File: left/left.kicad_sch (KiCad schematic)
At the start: 19 parts, among them J1 USB_C_Receptacle_IN, J2 USB_C_Receptacle_OUT, SW1 SW_Push, SW2 SW_SPDT, U1 STM32G0B1CBTx, U2 SRV05-4, U3 XC6206P332MR, U4 SRV05-4

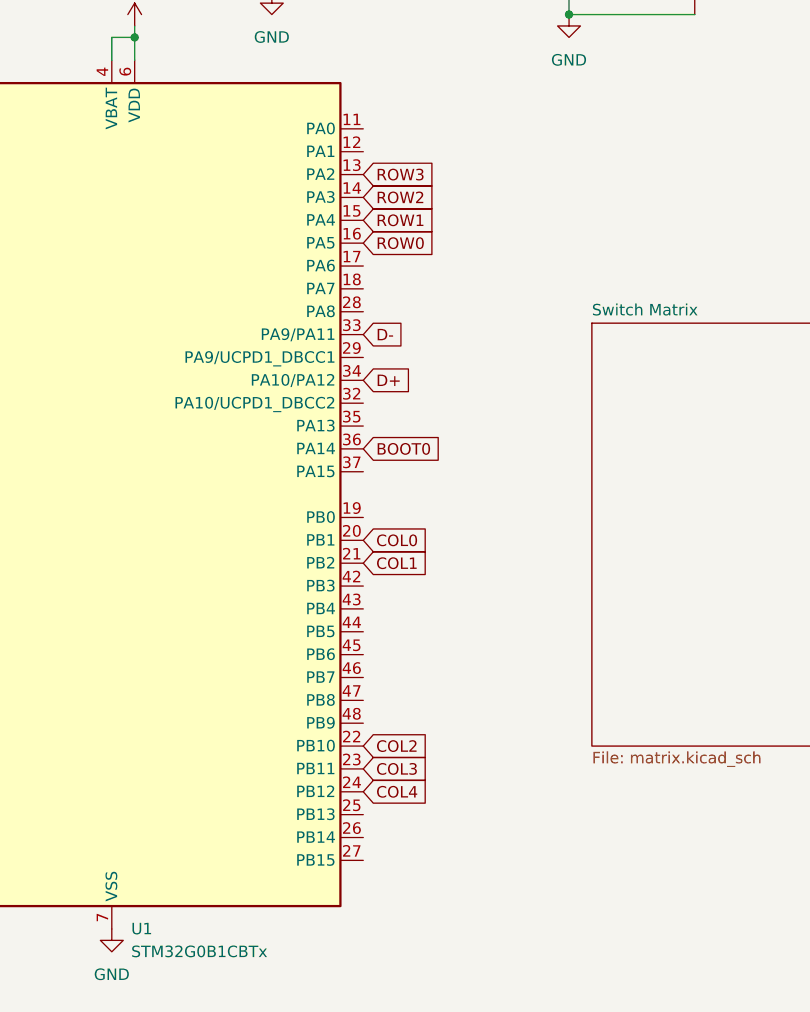
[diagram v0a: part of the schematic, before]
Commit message: should be done?
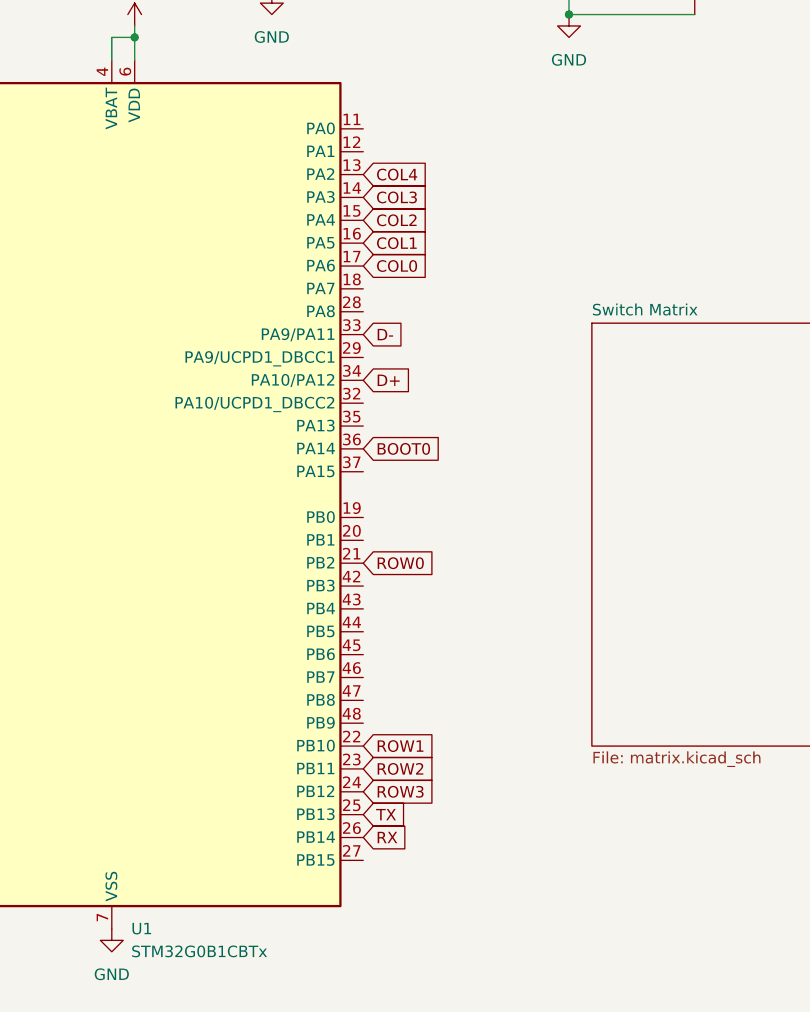
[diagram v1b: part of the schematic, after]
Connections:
- net COL0: now also U1.17 (PA6); no longer U1.20 (PB1)
- net COL1: now also U1.16 (PA5); no longer U1.21 (PB2)
- net COL2: now also U1.15 (PA4); no longer U1.22 (PB10)
- net COL3: now also U1.14 (PA3); no longer U1.23 (PB11)
- net COL4: now also U1.13 (PA2); no longer U1.24 (PB12)
- net ROW0: now also U1.21 (PB2); no longer U1.16 (PA5)
- net ROW1: now also U1.22 (PB10); no longer U1.15 (PA4)
- net ROW2: now also U1.23 (PB11); no longer U1.14 (PA3)
- net ROW3: now also U1.24 (PB12); no longer U1.13 (PA2)
- net RX: now also U1.26 (PB14)
- net TX: now also U1.25 (PB13)

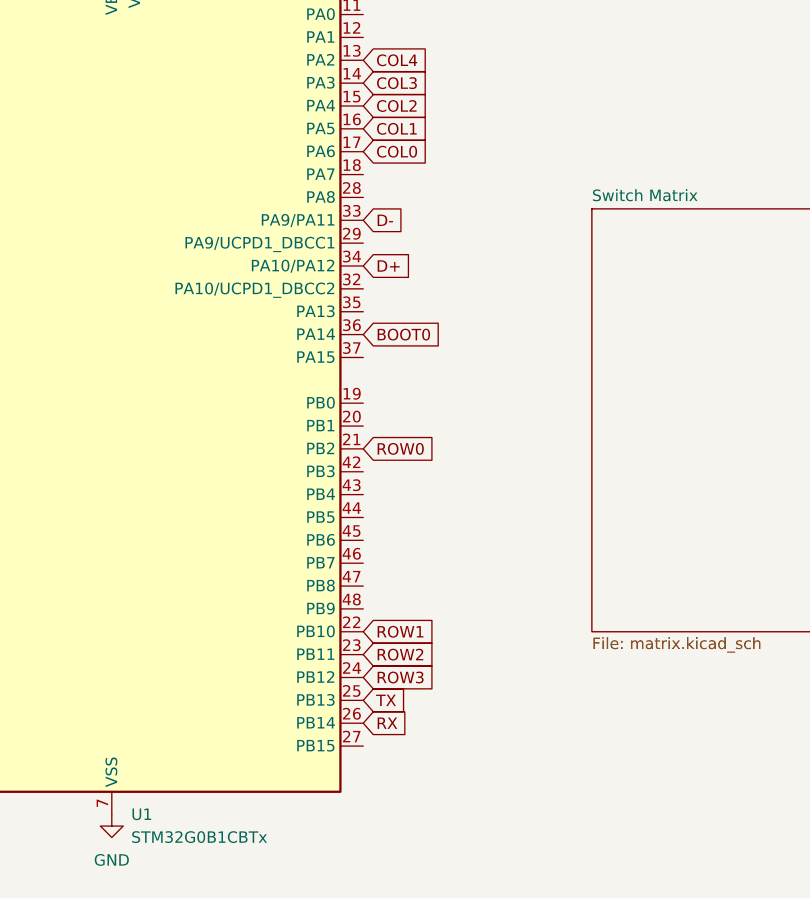
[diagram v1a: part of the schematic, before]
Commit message: fixed schematics
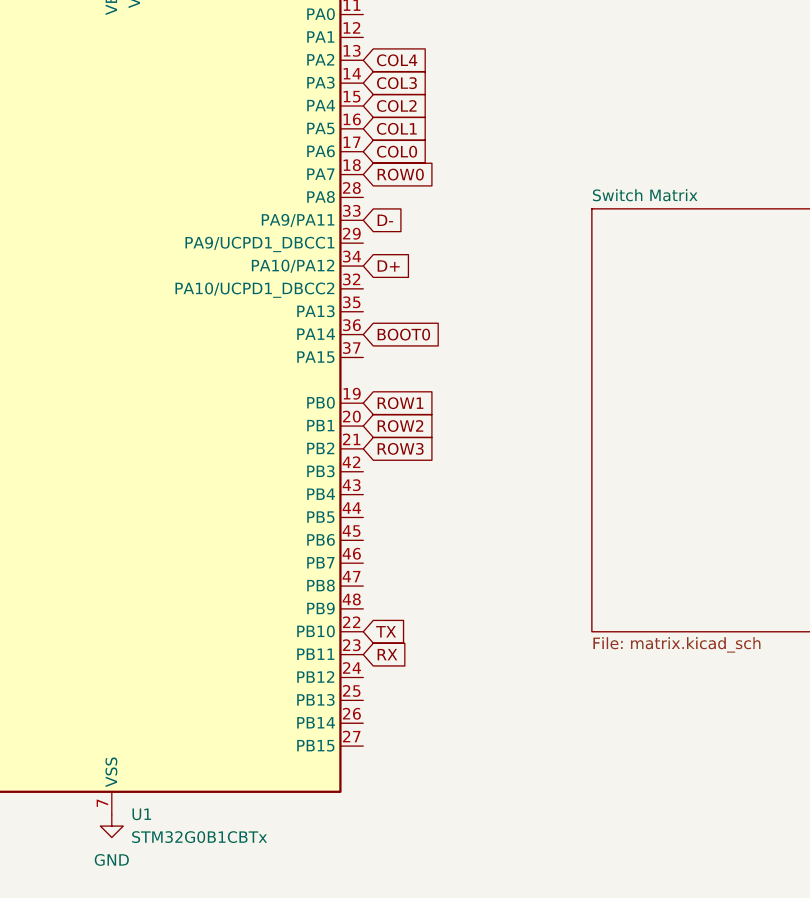
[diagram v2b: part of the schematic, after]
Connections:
- net ROW0: now also U1.18 (PA7); no longer U1.21 (PB2)
- net ROW1: now also U1.19 (PB0); no longer U1.22 (PB10)
- net ROW2: now also U1.20 (PB1); no longer U1.23 (PB11)
- net ROW3: now also U1.21 (PB2); no longer U1.24 (PB12)
- net RX: now also U1.23 (PB11); no longer U1.26 (PB14)
- net TX: now also U1.22 (PB10); no longer U1.25 (PB13)
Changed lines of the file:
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@@
 	(global_label "TX"
 		(shape input)
-		(at 111.76 120.65 0)
-		(fields_autoplaced yes)
-		(effects
-			(font
-				(size 1.27 1.27)
-			)
-			(justify left)
-		)
-		(property "Intersheetrefs" "${INTERSHEET_REFS}"
-			(at 116.9223 120.65 0)
+		(at 111.76 113.03 0)
+		(fields_autoplaced yes)
+		(effects
+			(font
+				(size 1.27 1.27)
+			)
+			(justify left)
+		)
+		(property "Intersheetrefs" "${INTERSHEET_REFS}"
+			(at 116.9223 113.03 0)
 			(hide yes)
 			(show_name no)
@@
 	(global_label "RX"
 		(shape input)
-		(at 111.76 123.19 0)
-		(fields_autoplaced yes)
-		(effects
-			(font
-				(size 1.27 1.27)
-			)
-			(justify left)
-		)
-		(property "Intersheetrefs" "${INTERSHEET_REFS}"
-			(at 117.2247 123.19 0)
+		(at 111.76 115.57 0)
+		(fields_autoplaced yes)
+		(effects
+			(font
+				(size 1.27 1.27)
+			)
+			(justify left)
+		)
+		(property "Intersheetrefs" "${INTERSHEET_REFS}"
+			(at 117.2247 115.57 0)
 			(hide yes)
 			(show_name no)
@@
 	(global_label "ROW1"
 		(shape input)
-		(at 111.76 113.03 0)
-		(fields_autoplaced yes)
-		(effects
-			(font
-				(size 1.27 1.27)
-			)
-			(justify left)
-		)
-		(property "Intersheetrefs" "${INTERSHEET_REFS}"
-			(at 120.0066 113.03 0)
+		(at 111.76 87.63 0)
+		(fields_autoplaced yes)
+		(effects
+			(font
+				(size 1.27 1.27)
+			)
+			(justify left)
+		)
+		(property "Intersheetrefs" "${INTERSHEET_REFS}"
+			(at 120.0066 87.63 0)
 			(hide yes)
 			(show_name no)
@@
 	(global_label "ROW3"
 		(shape input)
-		(at 111.76 118.11 0)
-		(fields_autoplaced yes)
-		(effects
-			(font
-				(size 1.27 1.27)
-			)
-			(justify left)
-		)
-		(property "Intersheetrefs" "${INTERSHEET_REFS}"
-			(at 120.0066 118.11 0)
+		(at 111.76 92.71 0)
+		(fields_autoplaced yes)
+		(effects
+			(font
+				(size 1.27 1.27)
+			)
+			(justify left)
+		)
+		(property "Intersheetrefs" "${INTERSHEET_REFS}"
+			(at 120.0066 92.71 0)
 			(hide yes)
 			(show_name no)
@@
 	(global_label "ROW0"
 		(shape input)
-		(at 111.76 92.71 0)
-		(fields_autoplaced yes)
-		(effects
-			(font
-				(size 1.27 1.27)
-			)
-			(justify left)
-		)
-		(property "Intersheetrefs" "${INTERSHEET_REFS}"
-			(at 120.0066 92.71 0)
+		(at 111.76 62.23 0)
+		(fields_autoplaced yes)
+		(effects
+			(font
+				(size 1.27 1.27)
+			)
+			(justify left)
+		)
+		(property "Intersheetrefs" "${INTERSHEET_REFS}"
+			(at 120.0066 62.23 0)
 			(hide yes)
 			(show_name no)
@@
 	(global_label "ROW2"
 		(shape input)
-		(at 111.76 115.57 0)
-		(fields_autoplaced yes)
-		(effects
-			(font
-				(size 1.27 1.27)
-			)
-			(justify left)
-		)
-		(property "Intersheetrefs" "${INTERSHEET_REFS}"
-			(at 120.0066 115.57 0)
-			(hide yes)
-			(show_name no)
+		(at 111.76 90.17 0)
+		(fields_autoplaced yes)
+		(effects
+			(font
+				(size 1.27 1.27)
+			)
+			(justify left)
+		)
+		(property "Intersheetrefs" "${INTERSHEET_REFS}"
+			(at 120.0066 90.17 0)
+			(hide yes)
+			(show_name no)

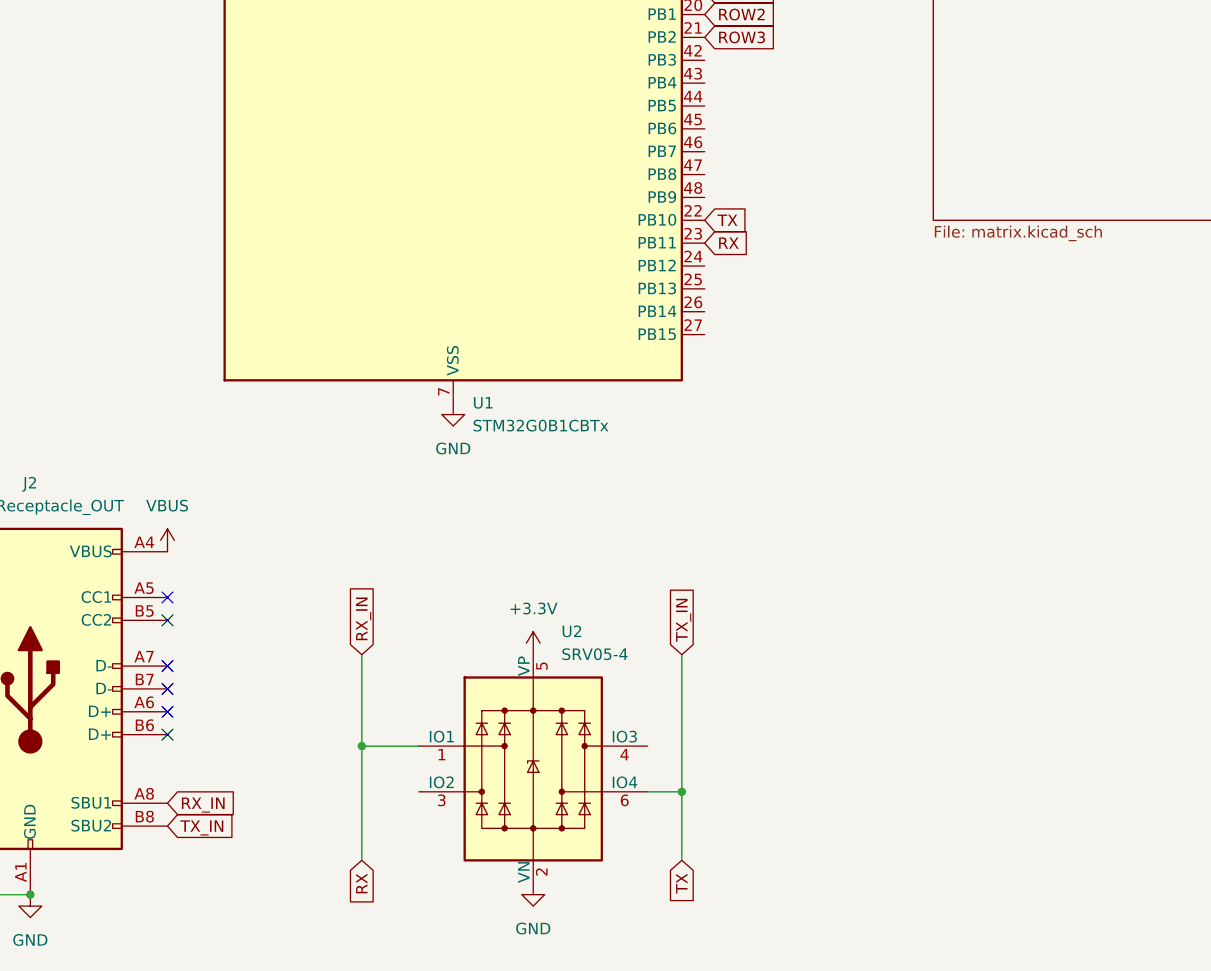
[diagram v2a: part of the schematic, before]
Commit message: v3 for the right side
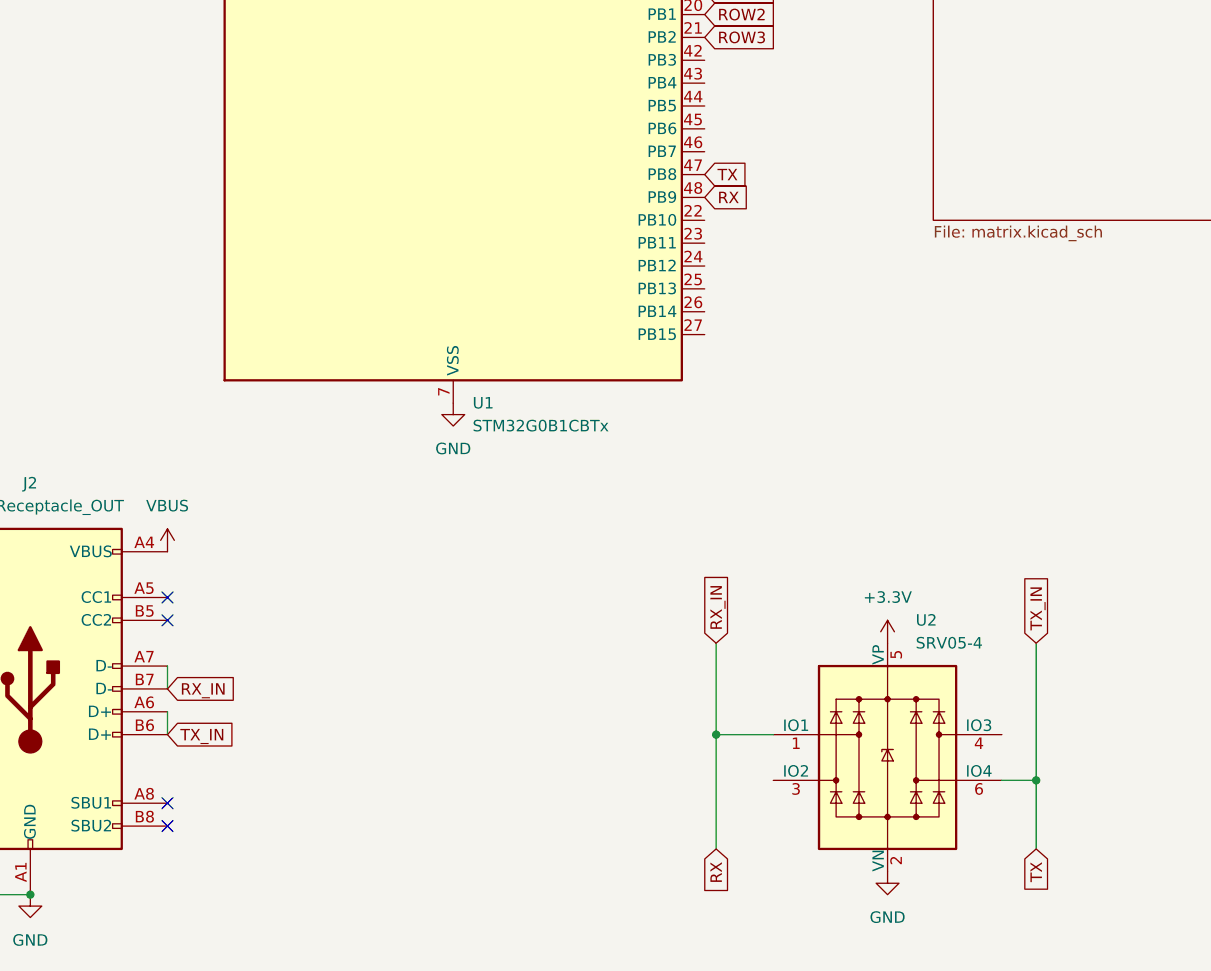
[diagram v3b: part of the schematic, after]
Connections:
- net RX: now also J2.A7 (D-), J2.B7 (D-), U1.48 (PB9); no longer J2.A8 (SBU1), U1.23 (PB11)
- net TX: now also J2.A6 (D+), J2.B6 (D+), U1.47 (PB8); no longer J2.B8 (SBU2), U1.22 (PB10)
- no-connect marks 8 -> 6
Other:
- moved on the sheet: U2
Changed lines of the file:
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@@
 	(paper "A4")
 	(junction
-		(at 73.66 171.45)
+		(at 113.03 170.18)
 		(diameter 0)
 		(color 0 0 0 0)
@@
 	)
 	(junction
-		(at 109.22 176.53)
+		(at 148.59 175.26)
 		(diameter 0)
 		(color 0 0 0 0)
@@
 	)
 	(no_connect
-		(at 52.07 165.1)
-	)
-	(no_connect
-		(at 52.07 162.56)
-	)
-	(no_connect
-		(at 52.07 170.18)
+		(at 52.07 180.34)
 	)
 	(no_connect
@@
 	)
 	(no_connect
-		(at 52.07 167.64)
+		(at 52.07 177.8)
 	)
 	(no_connect
@@
 	(wire
 		(pts
+			(xy 52.07 167.64) (xy 52.07 170.18)
+		)
+		(stroke
+			(width 0)
+			(type default)
+		)
+	)
+	(wire
+		(pts
 			(xy 101.6 21.59) (xy 109.22 21.59)
 		)
@@
 	(wire
 		(pts
-			(xy 73.66 171.45) (xy 80.01 171.45)
+			(xy 113.03 170.18) (xy 119.38 170.18)
 		)
 		(stroke
@@
 	(wire
 		(pts
-			(xy 73.66 171.45) (xy 73.66 184.15)
+			(xy 113.03 170.18) (xy 113.03 182.88)
 		)
 		(stroke
@@
 	(wire
 		(pts
-			(xy 109.22 161.29) (xy 109.22 176.53)
+			(xy 148.59 160.02) (xy 148.59 175.26)
 		)
 		(stroke
@@
 	(wire
 		(pts
-			(xy 105.41 176.53) (xy 109.22 176.53)
+			(xy 144.78 175.26) (xy 148.59 175.26)
 		)
 		(stroke
@@
 	(wire
 		(pts
-			(xy 73.66 161.29) (xy 73.66 171.45)
+			(xy 52.07 162.56) (xy 52.07 165.1)
+		)
+		(stroke
+			(width 0)
+			(type default)
+		)
+	)
+	(wire
+		(pts
+			(xy 113.03 160.02) (xy 113.03 170.18)
 		)
 		(stroke
@@
 	(wire
 		(pts
-			(xy 109.22 176.53) (xy 109.22 184.15)
+			(xy 148.59 175.26) (xy 148.59 182.88)
 		)
 		(stroke
@@
 	(global_label "RX_IN"
 		(shape input)
-		(at 73.66 161.29 90)
+		(at 113.03 160.02 90)
 		(fields_autoplaced yes)
 		(effects
@@
 		)
 		(property "Intersheetrefs" "${INTERSHEET_REFS}"
-			(at 73.66 152.9224 90)
+			(at 113.03 151.6524 90)
 			(hide yes)
 			(show_name no)
@@
 	(global_label "TX"
 		(shape input)
-		(at 111.76 113.03 0)
+		(at 111.76 107.95 0)
 		(fields_autoplaced yes)
 		(effects
@@
 		)
 		(property "Intersheetrefs" "${INTERSHEET_REFS}"
-			(at 116.9223 113.03 0)
+			(at 116.9223 107.95 0)
 			(hide yes)
 			(show_name no)
@@
 	(global_label "RX"
 		(shape input)
-		(at 111.76 115.57 0)
+		(at 111.76 110.49 0)
 		(fields_autoplaced yes)
 		(effects
@@
 		)
 		(property "Intersheetrefs" "${INTERSHEET_REFS}"
-			(at 117.2247 115.57 0)
+			(at 117.2247 110.49 0)
 			(hide yes)
 			(show_name no)
@@
 	(global_label "TX_IN"
 		(shape input)
-		(at 109.22 161.29 90)
+		(at 148.59 160.02 90)
 		(fields_autoplaced yes)
 		(effects
@@
 		)
 		(property "Intersheetrefs" "${INTERSHEET_REFS}"
-			(at 109.22 153.2248 90)
+			(at 148.59 151.9548 90)
 			(hide yes)
 			(show_name no)
@@
 	(global_label "TX_IN"
 		(shape input)
-		(at 52.07 180.34 0)
+		(at 52.07 170.18 0)
 		(fields_autoplaced yes)
 		(effects
@@
 		)
 		(property "Intersheetrefs" "${INTERSHEET_REFS}"
-			(at 60.1352 180.34 0)
+			(at 60.1352 170.18 0)
 			(hide yes)
 			(show_name no)
@@
 	(global_label "RX_IN"
 		(shape input)
-		(at 52.07 177.8 0)
+		(at 52.07 165.1 0)
 		(fields_autoplaced yes)
 		(effects
@@
 		)
 		(property "Intersheetrefs" "${INTERSHEET_REFS}"
-			(at 60.4376 177.8 0)
+			(at 60.4376 165.1 0)
 			(hide yes)
 			(show_name no)
@@
 	(global_label "TX"
 		(shape input)
-		(at 109.22 184.15 270)
+		(at 148.59 182.88 270)
 		(fields_autoplaced yes)
 		(effects
@@
 		)
 		(property "Intersheetrefs" "${INTERSHEET_REFS}"
-			(at 109.22 189.3123 90)
+			(at 148.59 188.0423 90)
 			(hide yes)
 			(show_name no)
@@
 	(global_label "RX"
 		(shape input)
-		(at 73.66 184.15 270)
+		(at 113.03 182.88 270)
 		(fields_autoplaced yes)
 		(effects
@@
 		)
 		(property "Intersheetrefs" "${INTERSHEET_REFS}"
-			(at 73.66 189.6147 90)
+			(at 113.03 188.3447 90)
 			(hide yes)
 			(show_name no)
@@
 	(symbol
 		(lib_id "power:GND")
-		(at 92.71 186.69 0)
+		(at 132.08 185.42 0)
 		(unit 1)
 		(body_style 1)
@@
 		(fields_autoplaced yes)
 		(property "Reference" "#PWR016"
-			(at 92.71 193.04 0)
+			(at 132.08 191.77 0)
 			(hide yes)
 			(show_name no)
@@
 		)
 		(property "Value" "GND"
-			(at 92.71 191.77 0)
+			(at 132.08 190.5 0)
 			(show_name no)
 			(do_not_autoplace no)
@@
 		)
 		(property "Footprint" ""
-			(at 92.71 186.69 0)
+			(at 132.08 185.42 0)
 			(hide yes)
 			(show_name no)
@@
 		)
 		(property "Datasheet" ""
-			(at 92.71 186.69 0)
+			(at 132.08 185.42 0)
 			(hide yes)
 			(show_name no)
@@
 		)
 		(property "Description" "Power symbol creates a global label with name \"GND\" , ground"
-			(at 92.71 186.69 0)
+			(at 132.08 185.42 0)
 			(hide yes)
 			(show_name no)
@@
 	(symbol
 		(lib_id "power:+3.3V")
-		(at 92.71 161.29 0)
+		(at 132.08 160.02 0)
 		(unit 1)
 		(body_style 1)
@@
 		(fields_autoplaced yes)
 		(property "Reference" "#PWR015"
-			(at 92.71 165.1 0)
+			(at 132.08 163.83 0)
 			(hide yes)
 			(show_name no)
@@
 		)
 		(property "Value" "+3.3V"
-			(at 92.71 156.21 0)
+			(at 132.08 154.94 0)
 			(show_name no)
 			(do_not_autoplace no)
@@
 		)
 		(property "Footprint" ""
-			(at 92.71 161.29 0)
+			(at 132.08 160.02 0)
 			(hide yes)
 			(show_name no)
@@
 		)
 		(property "Datasheet" ""
-			(at 92.71 161.29 0)
+			(at 132.08 160.02 0)
 			(hide yes)
 			(show_name no)
@@
 		)
 		(property "Description" "Power symbol creates a global label with name \"+3.3V\""
-			(at 92.71 161.29 0)
+			(at 132.08 160.02 0)
 			(hide yes)
 			(show_name no)
@@
 	(symbol
 		(lib_id "Power_Protection:SRV05-4")
-		(at 92.71 173.99 0)
+		(at 132.08 172.72 0)
 		(unit 1)
 		(body_style 1)
@@
 		(fields_autoplaced yes)
 		(property "Reference" "U2"
-			(at 95.8281 158.75 0)
+			(at 135.1981 157.48 0)
 			(show_name no)
 			(do_not_autoplace no)
@@
 		)
 		(property "Value" "SRV05-4"
-			(at 95.8281 161.29 0)
+			(at 135.1981 160.02 0)
 			(show_name no)
 			(do_not_autoplace no)
@@
 		)
 		(property "Footprint" "Package_TO_SOT_SMD:SOT-23-6"
-			(at 110.49 185.42 0)
+			(at 149.86 184.15 0)
 			(hide yes)
 			(show_name no)
@@
 		)
 		(property "Datasheet" "http://www.onsemi.com/pub/Collateral/SRV05-4-D.PDF"
-			(at 92.71 173.99 0)
+			(at 132.08 172.72 0)
 			(hide yes)
 			(show_name no)
@@
 		)
 		(property "Description" "ESD Protection Diodes with Low Clamping Voltage, SOT-23-6"
-			(at 92.71 173.99 0)
+			(at 132.08 172.72 0)
 			(hide yes)
 			(show_name no)
